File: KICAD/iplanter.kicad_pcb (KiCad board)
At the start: 2 copper layers, 64 x 71.5 mm, 5 parts, among them J1 Moisture Sensor, J2 Display, J3 DHT11, J4 Barrel_Jack_MountingPin, U2 WEMOS_D1_mini

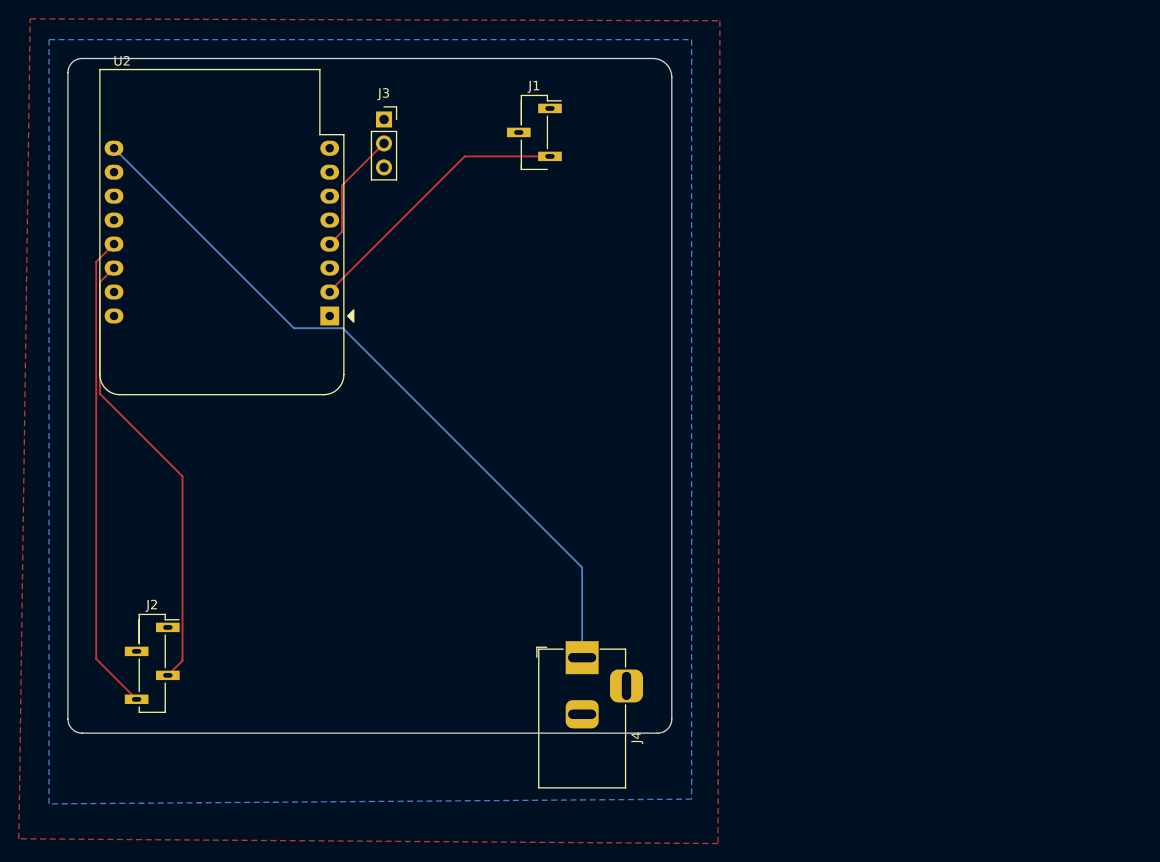
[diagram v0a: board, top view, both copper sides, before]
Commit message: Add files via upload
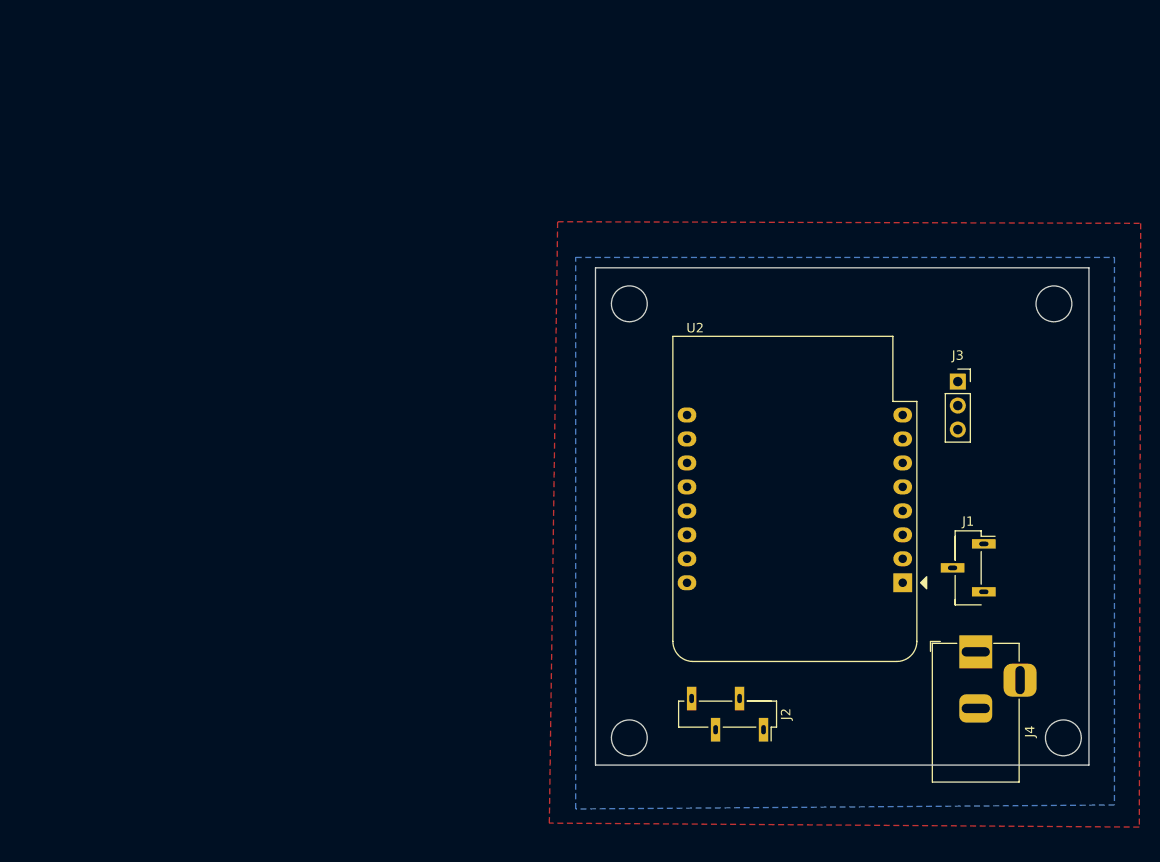
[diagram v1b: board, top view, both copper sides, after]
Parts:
- moved U2 67.0 mm to (154.0, 115.6)
- moved J3 66.9 mm to (159.8, 94.2)
- moved J1 65.1 mm to (160.9, 114.0)
- moved J2 61.2 mm to (135.4, 129.5), turned to -90 degrees
- moved J4 41.7 mm to (161.7, 122.9)
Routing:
- net Net-(U2-5V): track 77.6 -> 0.00 mm
- net /SDA: track 50.8 -> 0.00 mm
- net /SCL: track 48.1 -> 0.00 mm
- net /AOUT: track 29.3 -> 0.00 mm
- net Net-(J3-Pin_2): track 13.1 -> 0.00 mm
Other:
- board size 64 x 71.5 mm -> 52.3 x 52.7 mm
